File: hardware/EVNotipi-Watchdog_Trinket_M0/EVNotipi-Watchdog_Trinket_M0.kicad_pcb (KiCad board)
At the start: 2 copper layers, 25 x 34 mm, 13 parts, among them J1 Conn_M0_Left, J2 Conn_M0_Right, J3 Conn_Pi, J4 Conn_Pwr, J5 Conn_i2c, Q1 BS170, Q2 IRF5305, U1 TSR_2-2450

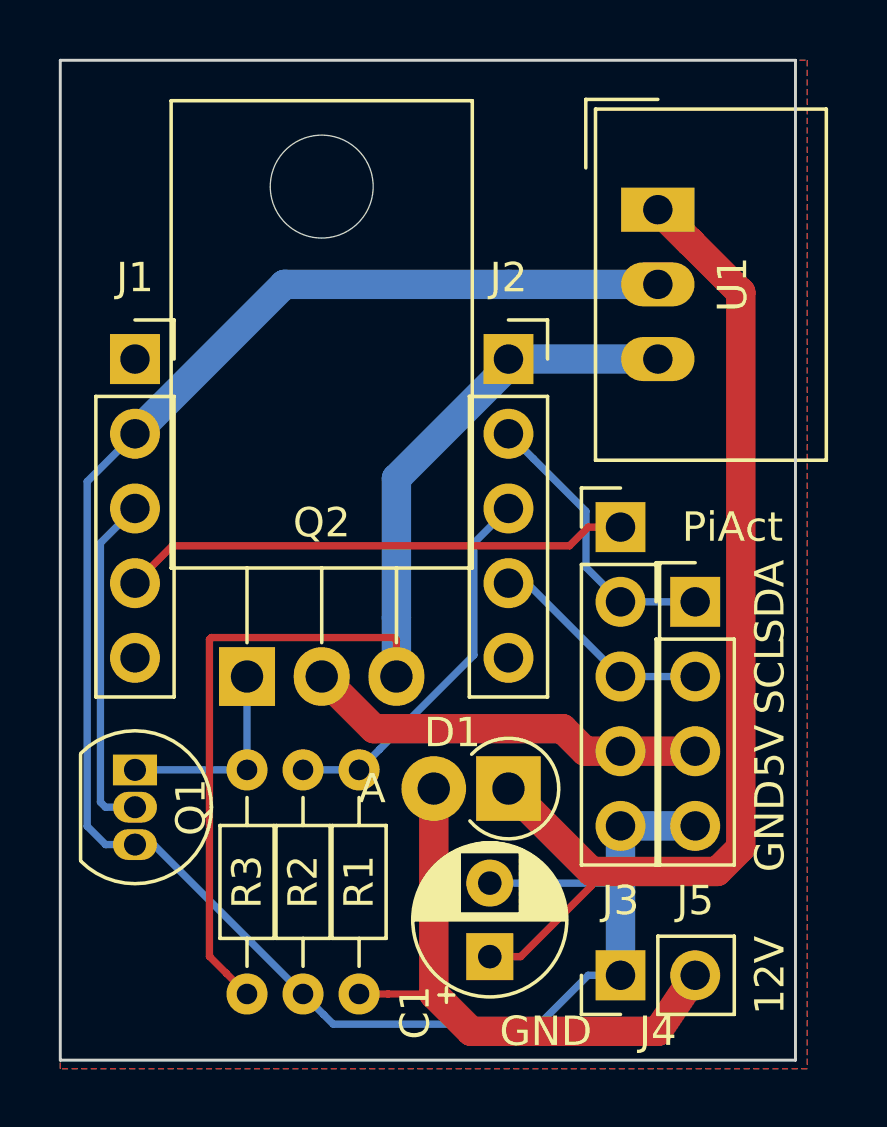
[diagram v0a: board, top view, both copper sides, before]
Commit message: updates to board
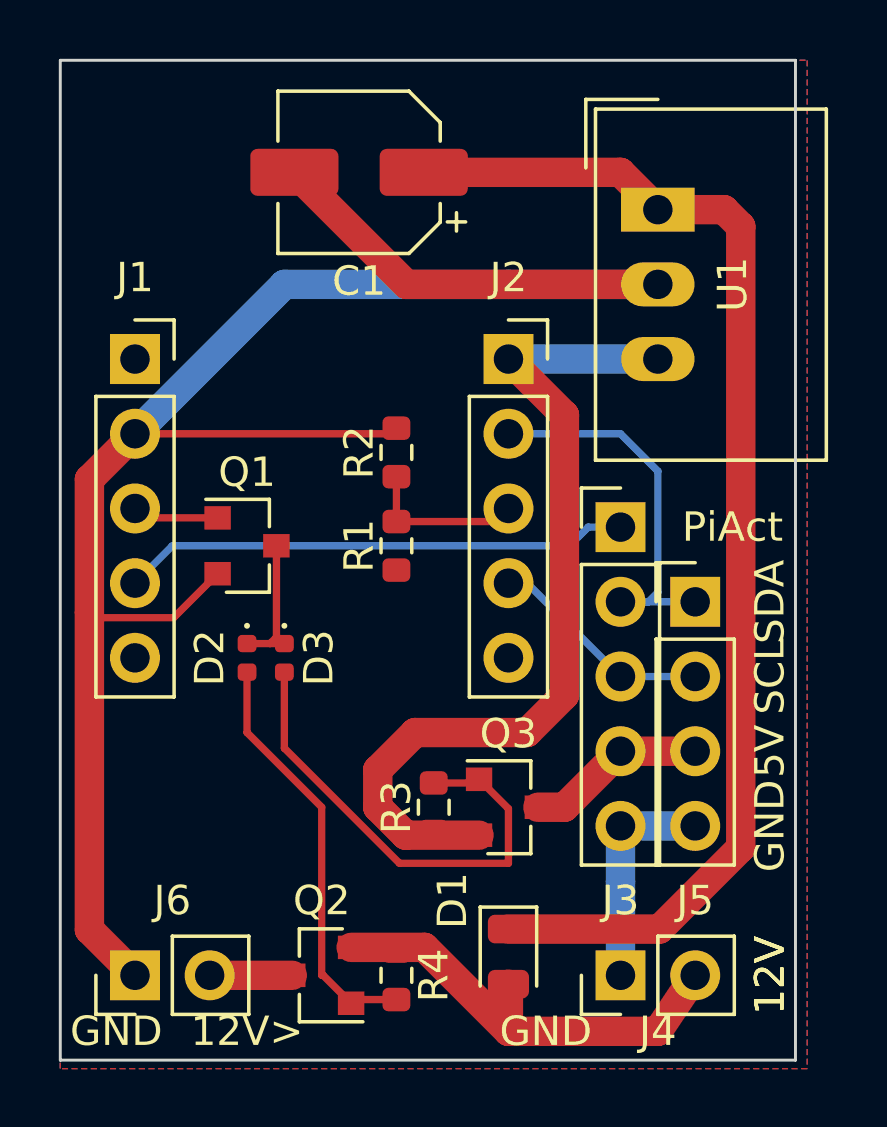
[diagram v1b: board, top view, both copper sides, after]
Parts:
- added D2: D_Schottky, Diode_SMD:D_0402_1005Metric, F.Cu at (61.0, 50.8)
- added D3: D_Schottky, Diode_SMD:D_0402_1005Metric, F.Cu at (62.2, 50.8)
- added J6: Conn_Pwr, Connector_PinHeader_2.54mm:PinHeader_1x02_P2.54mm_Vertical, F.Cu at (57.1, 61.6)
- added Q3: IRLML9301, Package_TO_SOT_SMD:SOT-23, F.Cu at (69.8, 55.9)
- added R4: R27K, Resistor_SMD:R_0603_1608Metric, F.Cu at (66.0, 61.6)
- C1: footprint Capacitor_THT:CP_Radial_D5.0mm_P2.50mm -> Capacitor_SMD:CP_Elec_5x3
- D1: footprint Diode_THT:D_DO-41_SOD81_P2.54mm_Vertical_AnodeUp -> Diode_SMD:D_0805_2012Metric
- Q1: value BS170 -> 2N7002; footprint Package_TO_SOT_THT:TO-92_Inline -> Package_TO_SOT_SMD:SOT-23
- Q2: value IRF5305 -> IRLML9301; footprint Package_TO_SOT_THT:TO-220-3_Horizontal_TabDown -> Package_TO_SOT_SMD:SOT-23
- R1, R2, R3: footprint Resistor_THT:R_Axial_DIN0204_L3.6mm_D1.6mm_P7.62mm_Horizontal -> Resistor_SMD:R_0603_1608Metric
- moved C1 27.0 mm to (64.8, 34.3), turned to 180 degrees
- moved R2 18.7 mm to (66.0, 43.8), turned to 270 degrees
- moved R1 15.3 mm to (66.0, 47.0)
- moved Q2 10.5 mm to (63.5, 61.6), turned to 180 degrees
- moved Q1 8.52 mm to (61.0, 47.0), turned to 0 degrees
- moved R3 6.48 mm to (67.3, 55.9)
- moved D1 5.72 mm to (69.8, 61.0), turned to 270 degrees
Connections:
- Q1 pad 1: Net-(Q1-Pad1) -> 5V_ENA
- Q1 pad 2: 5V_ENA -> GND
- Q1 pad 3: GND -> Net-(D2-Pad1)
- Q2 pad 1: Net-(Q1-Pad1) -> Net-(D2-Pad2)
- Q2 pad 2: VCC_Pi -> VCC12V
- Q2 pad 3: VCC5V -> 12V_OUT
- R3 pad 1: Net-(Q1-Pad1) -> Net-(D3-Pad2)
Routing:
- net Net-(D3-Pad2): track 0.00 -> 16.7 mm
- net Net-(D2-Pad2): track 0.00 -> 14.3 mm
- net 5V_ENA: track 11.7 -> 2.94 mm
- net GND: track 67.5 -> 75.2 mm
- net VCC_Pi: track 13.8 -> 6.14 mm
- net ADC: track 12.9 -> 5.71 mm
- net Net-(Q1-Pad1): track 6.98 -> 0.00 mm
- net VCC5V: track 37.7 -> 31.4 mm
- net Net-(D2-Pad1): track 0.00 -> 4.68 mm
- net Net-(C1-Pad1): track 37.7 -> 42.2 mm
- net SDA: track 9.83 -> 13.7 mm
- net VCC12V: track 20.0 -> 17.1 mm
- net 12V_OUT: track 0.00 -> 2.81 mm
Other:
- rule trace_min: 0.2 -> 10.2
- board text added: "12V>"
